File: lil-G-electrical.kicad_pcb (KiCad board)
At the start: 4 copper layers, 65 x 56 mm, 57 parts, among them J101 XT-60, J102 XT-60, J103 GPIO, J201 JST-SH, J202 JST-SH, J203 JST-SH, J204 JST-SH, Q101 STD26P3LLH6, SW101 PVA1EE, U101 MCP1415, U102 TPS565208, U201 A4950E, U202 A4950E, U203 A4950E, U204 A4950E

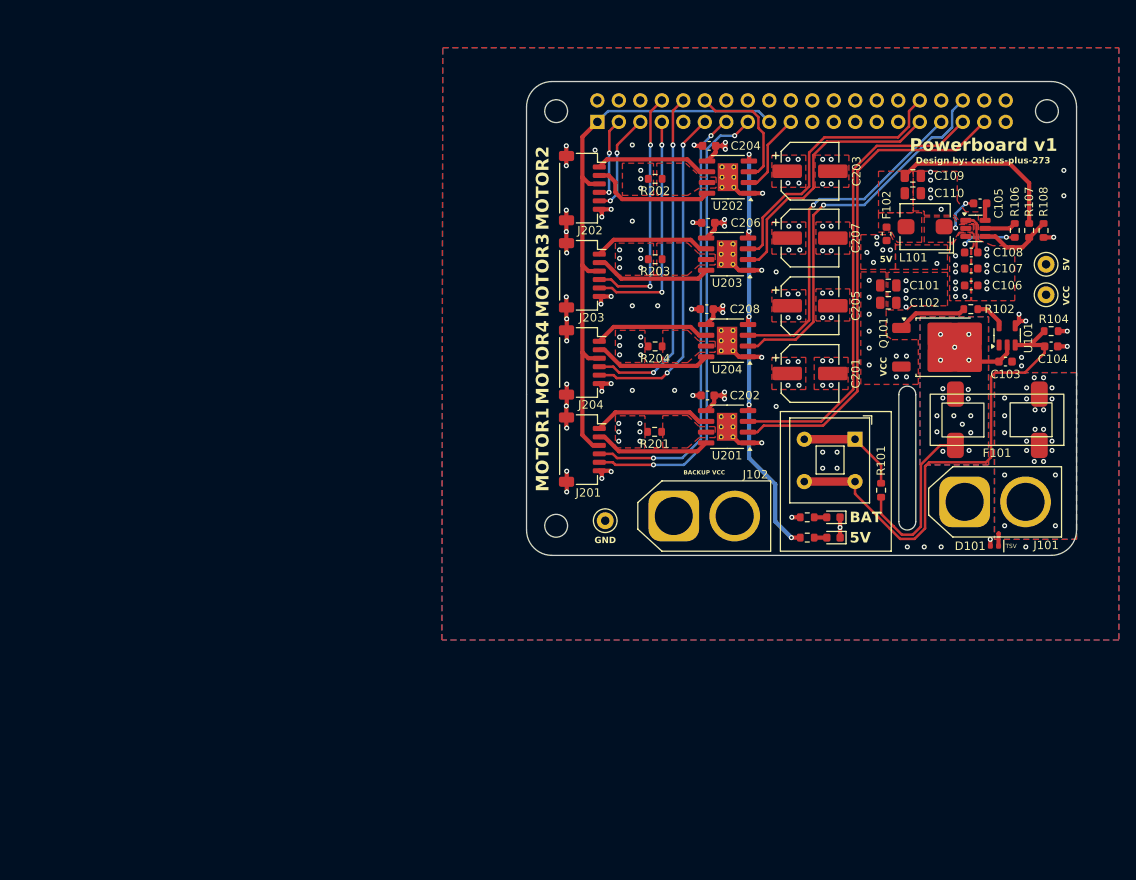
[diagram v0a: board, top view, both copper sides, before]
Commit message: version 2 done
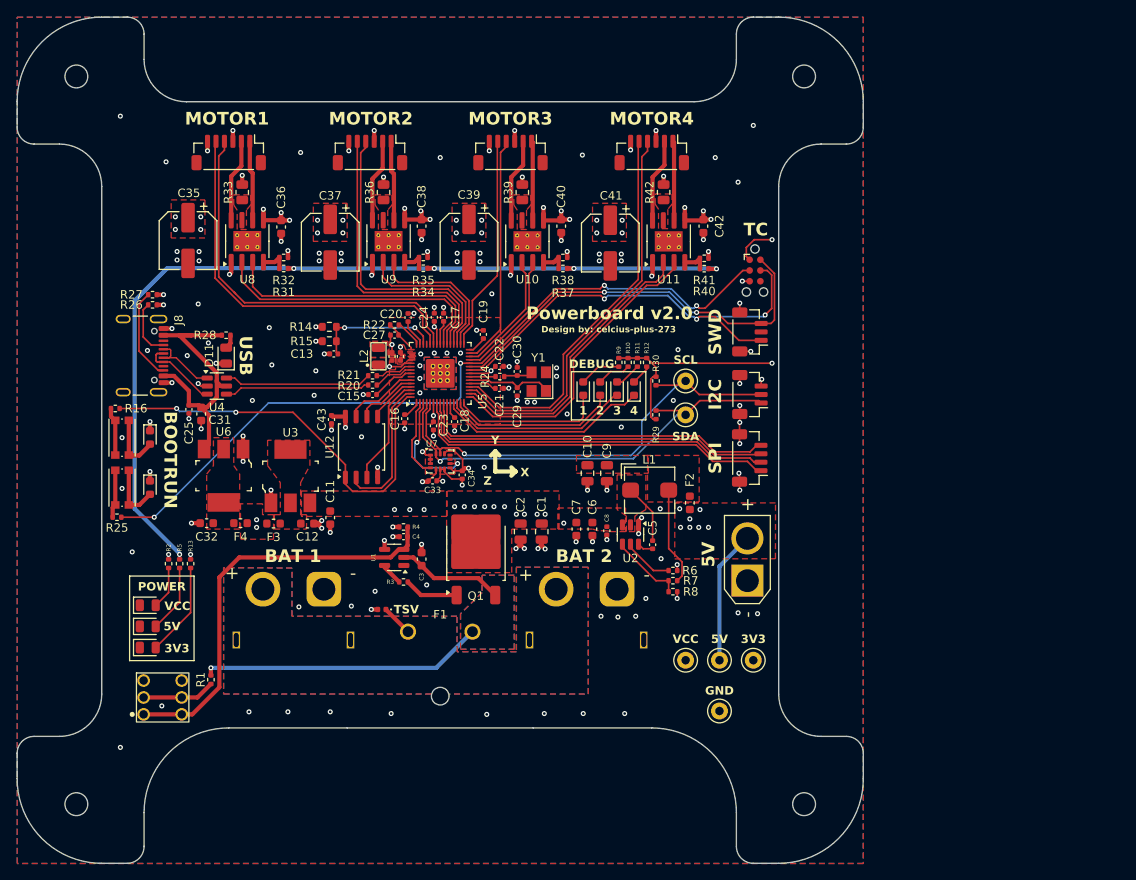
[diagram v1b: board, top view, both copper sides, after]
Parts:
- removed C101, C102, C109, C110: 22uF, Capacitor_SMD:C_0805_2012Metric
- removed C103, C106, C107: 10uF, Capacitor_SMD:C_0603_1608Metric
- removed C104, C105, C108: 0.1uF, Capacitor_SMD:C_0603_1608Metric
- removed C201, C203, C205, C207: 100uF, Capacitor_SMD:CP_Elec_6.3x7.7
- removed C202, C204, C206, C208: 0.22uF, Capacitor_SMD:C_0603_1608Metric
- removed D101: GG0402126R042P, Diode_SMD:D_0402_1005Metric
- removed D102, D103: GREEN, LED_SMD:LED_0603_1608Metric
- removed F101: 01000065Z, lilG_footprints:LittleFuse_Mini_100_SMD
- removed F102: 0686F5000, Fuse:Fuse_0603_1608Metric
- removed J101, J102: XT-60, Connector_AMASS:AMASS_XT60-M_1x02_P7.20mm_Vertical
- removed J103: GPIO, Connector_PinSocket_2.54mm:PinSocket_2x20_P2.54mm_Vertical
- removed J201, J202, J203, J204: JST-SH, Connector_JST:JST_SH_SM06B-SRSS-TB_1x06-1MP_P1.00mm_Horizontal
- removed L101: 3.3uH, Inductor_SMD:L_Bourns_SRP5030T
- removed Q101: STD26P3LLH6, Package_TO_SOT_SMD:TO-252-2
- removed R101, R103, R104, R106, R108: 10k, Resistor_SMD:R_0603_1608Metric
- removed R102: 22, Resistor_SMD:R_0603_1608Metric
- removed R105: 1k, Resistor_SMD:R_0603_1608Metric
- removed R107: 54.9k, Resistor_SMD:R_0603_1608Metric
- removed R201, R202, R203, R204: 500m, Resistor_SMD:R_0603_1608Metric
- removed SW101: PVA1EE, Button_Switch_THT:SW_Push_2P1T_Toggle_CK_PVA1xxH4xxxxxxV2
- removed TP101, TP102, TP103: TestPoint, TestPoint:TestPoint_Keystone_5000-5004_Miniature
- removed U101: MCP1415, Package_TO_SOT_SMD:SOT-23-5
- removed U102: TPS565208, Package_TO_SOT_SMD:SOT-23-6
- removed U201, U202, U203, U204: A4950E, Package_SO:SOIC-8-1EP_3.9x4.9mm_P1.27mm_EP2.41x3.3mm_ThermalVias
- added C1: 22uF, Capacitor_SMD:C_0805_2012Metric, F.Cu at (101.8, 97.2)
- added C10: 22uF, Capacitor_SMD:C_0805_2012Metric, F.Cu at (107.2, 90.3)
- added C11: 10uF, Capacitor_SMD:C_0603_1608Metric, F.Cu at (76.8, 95.5)
- added C12: 10uF, Capacitor_SMD:C_0603_1608Metric, F.Cu at (74.1, 96.2)
- added C13: 100n, Capacitor_SMD:C_0402_1005Metric, F.Cu at (77.2, 76.2)
- added C15: 100n, Capacitor_SMD:C_0402_1005Metric, F.Cu at (81.8, 81.0)
- added C16: 100n, Capacitor_SMD:C_0402_1005Metric, F.Cu at (85.6, 83.8)
- added C17: 100n, Capacitor_SMD:C_0402_1005Metric, F.Cu at (90.2, 71.9)
- added C18: 100n, Capacitor_SMD:C_0402_1005Metric, F.Cu at (91.5, 84.2)
- added C19: 100n, Capacitor_SMD:C_0402_1005Metric, F.Cu at (94.9, 73.9)
- added C2: 22uF, Capacitor_SMD:C_0805_2012Metric, F.Cu at (99.3, 97.2)
- added C20: 100n, Capacitor_SMD:C_0402_1005Metric, F.Cu at (86.0, 71.9)
- added C21: 100n, Capacitor_SMD:C_0402_1005Metric, F.Cu at (96.8, 80.3)
- added C22: 4.7u, Capacitor_SMD:C_0402_1005Metric, F.Cu at (96.8, 77.7)
- added C23: 100n, Capacitor_SMD:C_0402_1005Metric, F.Cu at (89.0, 84.7)
- added C24: 100n, Capacitor_SMD:C_0402_1005Metric, F.Cu at (89.1, 71.9)
- added C25: 100n, Capacitor_SMD:C_0402_1005Metric, F.Cu at (60.1, 82.7)
- added C26: 4.7u, Capacitor_SMD:C_0402_1005Metric, F.Cu at (84.1, 76.5)
- added C27: 4.7u, Capacitor_SMD:C_0402_1005Metric, F.Cu at (84.4, 74.0)
- added C28: 4.7u, Capacitor_SMD:C_0402_1005Metric, F.Cu at (85.1, 76.5)
- added C29: 15p, Capacitor_SMD:C_0402_1005Metric, F.Cu at (98.9, 80.7)
- added C3: 10uF, Capacitor_SMD:C_0603_1608Metric, F.Cu at (87.6, 100.4)
- added C30: 15p, Capacitor_SMD:C_0402_1005Metric, F.Cu at (98.9, 78.3)
- added C31: 10uF, Capacitor_SMD:C_0603_1608Metric, F.Cu at (61.5, 83.3)
- added C32: 10uF, Capacitor_SMD:C_0603_1608Metric, F.Cu at (62.2, 96.2)
- added C33: 100n, Capacitor_SMD:C_0402_1005Metric, F.Cu at (88.9, 91.2)
- added C34: 100n, Capacitor_SMD:C_0402_1005Metric, F.Cu at (92.4, 90.5)
- added C35: 100uF, Capacitor_SMD:CP_Elec_6.3x7.7, F.Cu at (60.0, 62.8)
- added C36: 0.22uF, Capacitor_SMD:C_0603_1608Metric, F.Cu at (71.0, 61.2)
- added C37: 100uF, Capacitor_SMD:CP_Elec_6.3x7.7, F.Cu at (76.8, 63.0)
- added C38: 0.22uF, Capacitor_SMD:C_0603_1608Metric, F.Cu at (87.6, 61.1)
- added C39: 100uF, Capacitor_SMD:CP_Elec_6.3x7.7, F.Cu at (93.2, 63.0)
- added C4: 100n, Capacitor_SMD:C_0402_1005Metric, F.Cu at (85.5, 97.8)
- added C40: 0.22uF, Capacitor_SMD:C_0603_1608Metric, F.Cu at (104.1, 61.1)
- added C41: 100uF, Capacitor_SMD:CP_Elec_6.3x7.7, F.Cu at (109.9, 63.1)
- added C42: 0.22uF, Capacitor_SMD:C_0603_1608Metric, F.Cu at (120.9, 61.1)
- added C43: 100n, Capacitor_SMD:C_0402_1005Metric, F.Cu at (77.0, 83.9)
- added C5: 100n, Capacitor_SMD:C_0402_1005Metric, F.Cu at (114.9, 98.7)
- added C6: 10uF, Capacitor_SMD:C_0603_1608Metric, F.Cu at (107.8, 96.9)
- added C7: 10uF, Capacitor_SMD:C_0603_1608Metric, F.Cu at (105.9, 96.9)
- added C8: 100n, Capacitor_SMD:C_0402_1005Metric, F.Cu at (109.5, 97.1)
- added C9: 22uF, Capacitor_SMD:C_0805_2012Metric, F.Cu at (109.5, 90.3)
- added D1: KT-0805G, LED_SMD:LED_0805_2012Metric, F.Cu at (55.2, 105.9)
- added D10: KT-0603R, LED_SMD:LED_0603_1608Metric, F.Cu at (55.5, 92.0)
- added D11: KT-0805G, LED_SMD:LED_0805_2012Metric, F.Cu at (64.5, 76.4)
- added D2: GG0402126R042P, Diode_SMD:D_0402_1005Metric, F.Cu at (82.9, 106.4)
- added D3: KT-0805G, LED_SMD:LED_0805_2012Metric, F.Cu at (55.2, 108.4)
- added D4: KT-0603W, LED_SMD:LED_0603_1608Metric, F.Cu at (106.7, 80.3)
- added D5: KT-0603W, LED_SMD:LED_0603_1608Metric, F.Cu at (108.7, 80.3)
- added D6: KT-0603W, LED_SMD:LED_0603_1608Metric, F.Cu at (110.7, 80.3)
- added D7: KT-0603W, LED_SMD:LED_0603_1608Metric, F.Cu at (112.7, 80.3)
- added D8: KT-0805G, LED_SMD:LED_0805_2012Metric, F.Cu at (55.2, 110.9)
- added D9: KT-0603R, LED_SMD:LED_0603_1608Metric, F.Cu at (55.5, 86.1)
- added F1: 01530007Z, lilG_footprints:LittleFuse_01530007Z, F.Cu at (89.8, 116.6)
- added F2: S0603-S-5.0A, Fuse:Fuse_0603_1608Metric, F.Cu at (119.3, 93.8)
- added F3: 0467001.NRHF, Fuse:Fuse_0603_1608Metric, F.Cu at (70.1, 96.2)
- added F4: 0467001.NRHF, Fuse:Fuse_0603_1608Metric, F.Cu at (66.2, 96.2)
- added J1: XT60-PW-M, Connector_AMASS:AMASS_XT60PW-M_1x02_P7.20mm_Horizontal, F.Cu at (76.0, 104.0)
- added J10: BM06B-SRSS-TB, Connector_JST:JST_SH_BM06B-SRSS-TB_1x06-1MP_P1.00mm_Vertical, F.Cu at (81.5, 52.4)
- added J11: BM06B-SRSS-TB, Connector_JST:JST_SH_BM06B-SRSS-TB_1x06-1MP_P1.00mm_Vertical, F.Cu at (98.1, 52.4)
- added J12: BM06B-SRSS-TB, Connector_JST:JST_SH_BM06B-SRSS-TB_1x06-1MP_P1.00mm_Vertical, F.Cu at (114.8, 52.4)
- added J2: XT30-U-M, Connector_AMASS:AMASS_XT30U-M_1x02_P5.0mm_Vertical, F.Cu at (126.1, 103.0)
- added J3: XT60-PW-M, Connector_AMASS:AMASS_XT60PW-M_1x02_P7.20mm_Horizontal, F.Cu at (110.7, 104.0)
- added J4: BM04B-SRSS-TB, Connector_JST:JST_SH_BM04B-SRSS-TB_1x04-1MP_P1.00mm_Vertical, F.Cu at (126.4, 88.5)
- added J5: BM03B-SRSS-TB, Connector_JST:JST_SH_BM03B-SRSS-TB_1x03-1MP_P1.00mm_Vertical, F.Cu at (126.4, 81.0)
- added J6: BM03B-SRSS-TB, Connector_JST:JST_SH_BM03B-SRSS-TB_1x03-1MP_P1.00mm_Vertical, F.Cu at (126.4, 73.6)
- added J7: TC2030-NL, Connector:Tag-Connect_TC2030-IDC-NL_2x03_P1.27mm_Vertical, F.Cu at (127.0, 66.3)
- added J8: TYPE-C16PIN, Connector_USB:USB_C_Receptacle_GCT_USB4105-xx-A_16P_TopMnt_Horizontal, F.Cu at (53.4, 76.4)
- added J9: BM06B-SRSS-TB, Connector_JST:JST_SH_BM06B-SRSS-TB_1x06-1MP_P1.00mm_Vertical, F.Cu at (64.8, 52.4)
- added L1: SRP5030T-3R3M, Inductor_SMD:L_Bourns_SRP5030T, F.Cu at (114.5, 92.3)
- added L2: AOTA-B201610S3R3-101-T, lilG_footprints:L_0806, F.Cu at (82.5, 76.5)
- added MH4: MountingHole_2.7mm_M2.5, MountingHole:MountingHole_2.7mm_M2.5, F.Cu at (132.8, 129.4)
- added Q1: 40P30, Package_TO_SOT_SMD:TO-252-2, F.Cu at (94.0, 99.7)
- added R1: 10k, Resistor_SMD:R_0402_1005Metric, F.Cu at (62.7, 114.7)
- added R10: 1k, Resistor_SMD:R_0402_1005Metric, F.Cu at (112.0, 77.2)
- added R11: 1k, Resistor_SMD:R_0402_1005Metric, F.Cu at (113.1, 77.2)
- added R12: 1k, Resistor_SMD:R_0402_1005Metric, F.Cu at (114.2, 77.2)
- added R13: 1k, Resistor_SMD:R_0402_1005Metric, F.Cu at (60.3, 101.0)
- added R14: 300k, Resistor_SMD:R_0603_1608Metric, F.Cu at (76.7, 73.0)
- added R15: 100k, Resistor_SMD:R_0603_1608Metric, F.Cu at (76.7, 74.7)
- added R16: 1k, Resistor_SMD:R_0402_1005Metric, F.Cu at (51.4, 82.6)
- added R2: 4.7k, Resistor_SMD:R_0402_1005Metric, F.Cu at (57.7, 101.0)
- added R20: 27, Resistor_SMD:R_0402_1005Metric, F.Cu at (81.8, 79.9)
- added R21: 27, Resistor_SMD:R_0402_1005Metric, F.Cu at (81.8, 78.8)
- added R22: 33, Resistor_SMD:R_0402_1005Metric, F.Cu at (84.4, 72.8)
- added R24: 1k, Resistor_SMD:R_0402_1005Metric, F.Cu at (96.8, 78.9)
- added R25: 1k, Resistor_SMD:R_0402_1005Metric, F.Cu at (51.6, 95.5)
- added R26: 5.1k, Resistor_SMD:R_0402_1005Metric, F.Cu at (55.8, 70.4)
- added R27: 5.1k, Resistor_SMD:R_0402_1005Metric, F.Cu at (55.8, 69.2)
- added R28: 1k, Resistor_SMD:R_0402_1005Metric, F.Cu at (64.5, 74.0)
- added R29: 4.7k, Resistor_SMD:R_0402_1005Metric, F.Cu at (115.3, 83.4)
- added R3: 22, Resistor_SMD:R_0402_1005Metric, F.Cu at (85.5, 103.1)
- added R30: 4.7k, Resistor_SMD:R_0402_1005Metric, F.Cu at (115.3, 79.4)
- added R31: 200k, Resistor_SMD:R_0402_1005Metric, F.Cu at (71.3, 66.1)
- added R32: 50k, Resistor_SMD:R_0402_1005Metric, F.Cu at (71.3, 64.8)
- added R33: RL10FTNR100, Resistor_SMD:R_0805_2012Metric, F.Cu at (66.4, 57.1)
- added R34: 200k, Resistor_SMD:R_0402_1005Metric, F.Cu at (87.8, 66.1)
- added R35: 50k, Resistor_SMD:R_0402_1005Metric, F.Cu at (87.8, 64.8)
- added R36: RL10FTNR100, Resistor_SMD:R_0805_2012Metric, F.Cu at (83.1, 57.1)
- added R37: 200k, Resistor_SMD:R_0402_1005Metric, F.Cu at (104.3, 66.1)
- added R38: 50k, Resistor_SMD:R_0402_1005Metric, F.Cu at (104.3, 64.8)
- added R39: RL10FTNR100, Resistor_SMD:R_0805_2012Metric, F.Cu at (99.5, 57.1)
- added R4: 10k, Resistor_SMD:R_0402_1005Metric, F.Cu at (85.5, 96.6)
- added R40: 200k, Resistor_SMD:R_0402_1005Metric, F.Cu at (121.0, 66.1)
- added R41: 50k, Resistor_SMD:R_0402_1005Metric, F.Cu at (121.0, 64.9)
- added R42: RL10FTNR100, Resistor_SMD:R_0805_2012Metric, F.Cu at (116.2, 57.1)
- added R5: 1k, Resistor_SMD:R_0402_1005Metric, F.Cu at (59.0, 101.0)
- added R6: 10k, Resistor_SMD:R_0402_1005Metric, F.Cu at (117.3, 101.8)
- added R7: 54.9k, Resistor_SMD:R_0402_1005Metric, F.Cu at (117.3, 103.0)
- added R8: 10k, Resistor_SMD:R_0402_1005Metric, F.Cu at (117.3, 104.3)
- added R9: 1k, Resistor_SMD:R_0402_1005Metric, F.Cu at (110.9, 77.2)
- added SW1: 5.8 ZSGT, lilG_footprints:5.8_ZSGT, F.Cu at (57.0, 116.8)
- added SW2: KMR2, Button_Switch_SMD:SW_Push_1P1T_NO_CK_KMR2, F.Cu at (52.2, 86.1)
- added SW3: KMR2, Button_Switch_SMD:SW_Push_1P1T_NO_CK_KMR2, F.Cu at (52.2, 92.0)
- added TP1: 5001, TestPoint:TestPoint_Keystone_5000-5004_Miniature, F.Cu at (118.8, 112.4)
- added TP2: 5001, TestPoint:TestPoint_Keystone_5000-5004_Miniature, F.Cu at (122.8, 118.4)
- added TP3: 5001, TestPoint:TestPoint_Keystone_5000-5004_Miniature, F.Cu at (122.8, 112.4)
- added TP4: 5001, TestPoint:TestPoint_Keystone_5000-5004_Miniature, F.Cu at (118.8, 79.4)
- added TP5: 5001, TestPoint:TestPoint_Keystone_5000-5004_Miniature, F.Cu at (118.8, 83.4)
- added TP6: 5001, TestPoint:TestPoint_Keystone_5000-5004_Miniature, F.Cu at (126.8, 112.4)
- added U1: MCP1415, Package_TO_SOT_SMD:SOT-23-5, F.Cu at (84.4, 100.2)
- added U10: A4950E, Package_SO:SOIC-8-1EP_3.9x4.9mm_P1.27mm_EP2.41x3.3mm_ThermalVias, F.Cu at (100.1, 62.9)
- added U11: A4950E, Package_SO:SOIC-8-1EP_3.9x4.9mm_P1.27mm_EP2.41x3.3mm_ThermalVias, F.Cu at (116.8, 62.9)
- added U12: W25Q128JVS, Package_SO:SOIC-8_5.23x5.23mm_P1.27mm, F.Cu at (80.5, 87.2)
- added U2: TPS565208, Package_TO_SOT_SMD:SOT-23-6, F.Cu at (112.3, 97.5)
- added U3: NCP1117ST33T3G, digikey-footprints:SOT-223, F.Cu at (72.1, 90.6)
- added U4: USBLC6-2SC6, Package_TO_SOT_SMD:SOT-23-6, F.Cu at (63.4, 80.0)
- added U5: RP2350A, lilG_footprints:QFN-60-1EP_7x7mm_P0.4mm_EP3.4x3.4mm_ThermalVias, F.Cu at (89.8, 78.5)
- added U6: NCP1117ST33T3G, digikey-footprints:SOT-223, F.Cu at (64.2, 90.6)
- added U7: LSM6DSM, Package_LGA:LGA-14_3x2.5mm_P0.5mm_LayoutBorder3x4y, F.Cu at (89.8, 88.9)
- added U8: A4950E, Package_SO:SOIC-8-1EP_3.9x4.9mm_P1.27mm_EP2.41x3.3mm_ThermalVias, F.Cu at (67.0, 62.9)
- added U9: A4950E, Package_SO:SOIC-8-1EP_3.9x4.9mm_P1.27mm_EP2.41x3.3mm_ThermalVias, F.Cu at (83.7, 62.9)
- added Y1: ABM8-272-T3, Crystal:Crystal_SMD_Abracon_ABM8G-4Pin_3.2x2.5mm, F.Cu at (101.5, 79.5)
- moved MH2 140.9 mm to (46.8, 129.4)
- moved MH3 60.6 mm to (132.8, 43.4)
- moved MH1 56.8 mm to (46.8, 43.4)
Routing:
- net +3V3: track 68.5 -> 329.4 mm, vias 0 -> 19
- net /rp2350a/~{RESET}: track 0.00 -> 91.2 mm, vias 0 -> 4
- net /M1_DIR: track 58.3 -> 0.00 mm
- net /rp2350a/SWCLK: track 0.00 -> 55.8 mm, vias 0 -> 3
- net /M1_PWM: track 55.3 -> 0.00 mm
- net /I2C_SCL: track 0.00 -> 55.0 mm, vias 0 -> 1
- net /I2C_SDA: track 0.00 -> 52.7 mm, vias 0 -> 1
- net +5V: track 109.9 -> 161.5 mm
- net /rp2350a/BOOTSEL: track 0.00 -> 49.3 mm, vias 0 -> 2
- net /rp2350a/SWDIO: track 0.00 -> 49.2 mm, vias 0 -> 2
- net /VBAT_FUSED: track 0.00 -> 46.2 mm, vias 0 -> 1
- net /M4_DIR: track 45.9 -> 0.00 mm, vias 1 -> 0
- net /SPI_RX: track 0.00 -> 43.8 mm
- net /SPI_CSn: track 0.00 -> 42.9 mm
- net /SPI_SCK: track 0.00 -> 42.2 mm
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- added copper zone on F.Cu, net +1V1
- added copper zone on In2.Cu, net +1V1
- added copper zone on F.Cu, net +3V3
- added copper zone on In2.Cu, net +3V3
- added copper zone on F.Cu, net /5V_RAW
- added copper zone on B.Cu, net /BAT_1
- added copper zone on F.Cu, net /BAT_1
- added copper zone on B.Cu, net /VBAT_FUSED
- added copper zone on F.Cu, net /VBAT_FUSED
- added copper zone on F.Cu, net /rp2350a/VREG_LX
- added copper zone on F.Cu, net Net-(C12-Pad1)
- added copper zone on F.Cu, net Net-(C32-Pad1)
- added copper zone on F.Cu, net Net-(U10-LSS)
- added copper zone on F.Cu, net Net-(U11-LSS)
- added copper zone on F.Cu, net Net-(U2-SW)
- added copper zone on F.Cu, net Net-(U8-LSS)
- added copper zone on F.Cu, net Net-(U9-LSS)
- removed copper zone on F.Cu, net Net-(C109-Pad1)
- removed copper zone on B.Cu, net Net-(D101-K)
- removed copper zone on F.Cu, net Net-(D101-K)
- removed copper zone on B.Cu, net Net-(Q101-D)
- removed copper zone on F.Cu, net Net-(Q101-D)
- removed copper zone on F.Cu, net Net-(U102-SW)
- removed copper zone on F.Cu, net Net-(U201-LSS)
- removed copper zone on F.Cu, net Net-(U202-LSS)
- removed copper zone on F.Cu, net Net-(U203-LSS)
- removed copper zone on F.Cu, net Net-(U204-LSS)
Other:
- board size 65 x 56 mm -> 100 x 100 mm
- board text added: "1"
- board text added: "2"
- board text added: "3"
- board text added: "3V3"
- board text added: "4"
- board text added: "BAT 1"
- board text added: "BAT 2"
- board text added: "BOOT"
- board text added: "DEBUG"
- board text added: "DOWN"
- board text added: "I2C"
- board text added: "POWER"
- board text added: "Powerboard v2.0"
- board text added: "RUN"
- board text added: "SCL"
- board text added: "SDA"
- board text added: "SPI"
- board text added: "SWD"
- board text added: "TC"
- board text added: "UP"
- board text added: "X"
- board text added: "Y"
- board text added: "Z"
- board text removed: "BACKUP VCC"
- board text removed: "BAT"
- board text removed: "CAMERA (OPTIONAL)"
- board text removed: "DISPLAY (OPTIONAL)"
- board text removed: "Extend PCB edge 0.5mm if using SMT header"
- board text removed: "PoE"
- board text removed: "Powerboard v1"
- board text removed: "RJ45"
